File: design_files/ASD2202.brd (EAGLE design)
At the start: 22.5 x 21.3 mm, 21 parts, among them J1 DF12-32-DP, J2 DF12-32-DS, U1 XC6217A332MR-G, U2 24FC1025T-I/SN, U4 TXB0104, U5 W25Q80DVSNIG, MB85RS1MTPNF, 2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

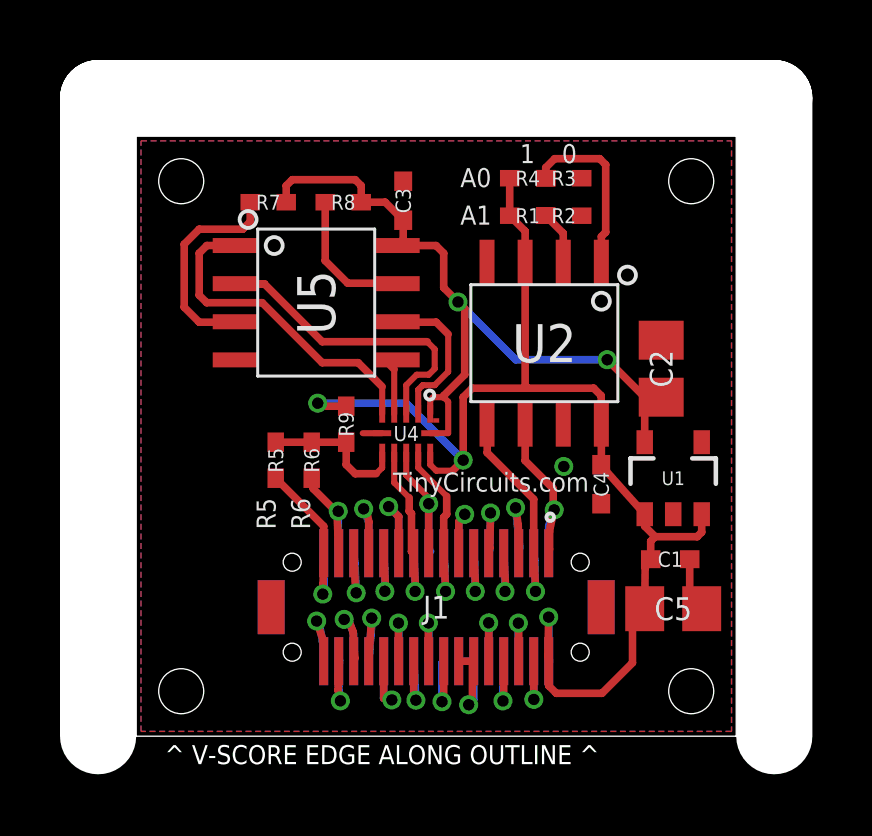
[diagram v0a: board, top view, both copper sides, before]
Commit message: update format
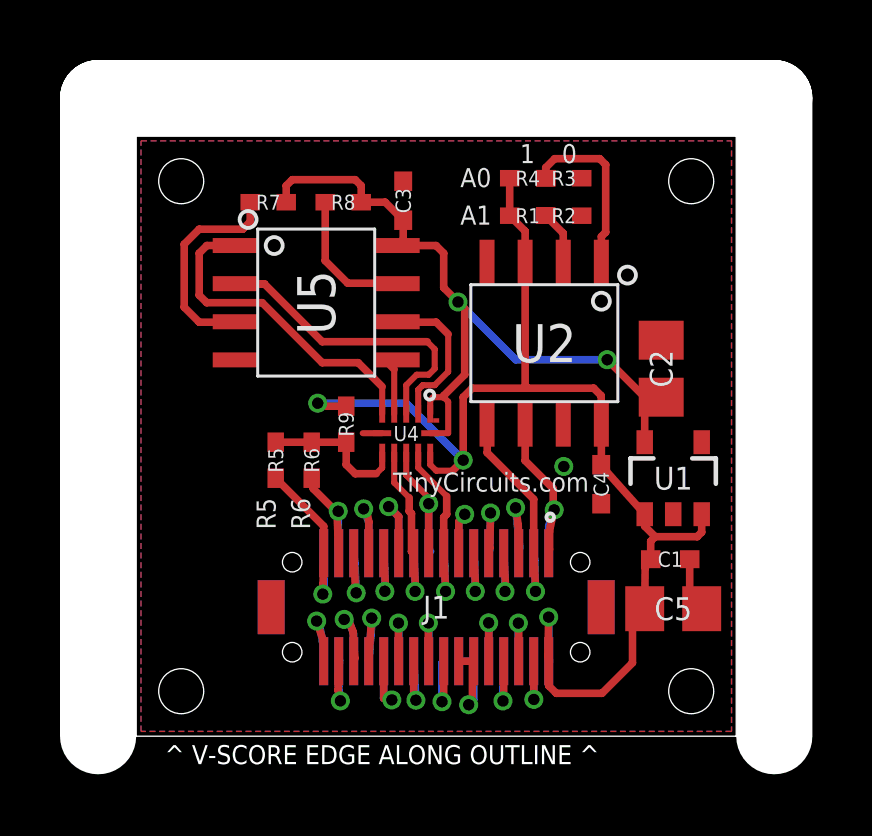
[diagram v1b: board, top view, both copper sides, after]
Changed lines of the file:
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@@
 <setting verticaltext="up"/>
 </settings>
-<grid distance="0.05" unitdist="mm" unit="mm" style="lines" multiple="1" display="yes" altdistance="0.025" altunitdist="inch" altunit="inch"/>
+<grid distance="0.1" unitdist="mm" unit="mm" style="lines" multiple="1" display="yes" altdistance="0.025" altunitdist="inch" altunit="inch"/>
 <layers>
 <layer number="1" name="Top" color="4" fill="1" visible="yes" active="yes"/>
@@
 <layer number="54" name="bGND_GNDA" color="7" fill="1" visible="yes" active="yes"/>
 <layer number="56" name="wert" color="7" fill="1" visible="yes" active="yes"/>
+<layer number="57" name="tCAD" color="7" fill="1" visible="no" active="no"/>
+<layer number="58" name="bCAD" color="7" fill="1" visible="no" active="no"/>
+<layer number="59" name="Invisible" color="7" fill="1" visible="no" active="no"/>
+<layer number="61" name="stand" color="7" fill="1" visible="no" active="no"/>
+<layer number="90" name="Modules" color="5" fill="1" visible="yes" active="yes"/>
 <layer number="91" name="Nets" color="2" fill="1" visible="no" active="no"/>
 <layer number="92" name="Busses" color="1" fill="1" visible="no" active="no"/>
@@
 <layer number="97" name="Info" color="7" fill="1" visible="no" active="no"/>
 <layer number="98" name="Guide" color="6" fill="1" visible="no" active="no"/>
+<layer number="99" name="SpiceOrder" color="5" fill="1" visible="no" active="no"/>
 <layer number="100" name="Muster" color="7" fill="1" visible="yes" active="yes"/>
 <layer number="101" name="Patch_Top" color="7" fill="1" visible="yes" active="yes"/>
@@
 <layer number="111" name="tGTest" color="4" fill="1" visible="no" active="no"/>
 <layer number="112" name="bGTest" color="1" fill="1" visible="no" active="no"/>
+<layer number="113" name="HENWAY_PKG" color="12" fill="1" visible="yes" active="yes"/>
+<layer number="114" name="50_Electronics_Plate" color="7" fill="1" visible="yes" active="yes"/>
+<layer number="115" name="henwayRES" color="5" fill="1" visible="yes" active="yes"/>
 <layer number="116" name="Patch_BOT" color="7" fill="1" visible="yes" active="yes"/>
 <layer number="117" name="mPads" color="7" fill="1" visible="no" active="no"/>
@@
 <layer number="151" name="HeatSink" color="7" fill="1" visible="yes" active="yes"/>
 <layer number="152" name="mbDocu" color="7" fill="1" visible="no" active="no"/>
+<layer number="153" name="FabDoc1" color="6" fill="1" visible="no" active="no"/>
+<layer number="154" name="FabDoc2" color="2" fill="1" visible="no" active="no"/>
+<layer number="155" name="FabDoc3" color="7" fill="15" visible="no" active="no"/>
+<layer number="156" name="bCapacitor" color="7" fill="1" visible="no" active="yes"/>
+<layer number="157" name="tResistor" color="7" fill="1" visible="no" active="yes"/>
+<layer number="158" name="bResistor" color="7" fill="1" visible="no" active="yes"/>
+<layer number="159" name="henwayCAP" color="13" fill="1" visible="yes" active="yes"/>
 <layer number="191" name="mNets" color="7" fill="1" visible="no" active="no"/>
 <layer number="192" name="mBusses" color="7" fill="1" visible="no" active="no"/>
@@
 <layer number="223" name="223bmp" color="7" fill="1" visible="yes" active="yes"/>
 <layer number="224" name="224bmp" color="7" fill="1" visible="yes" active="yes"/>
+<layer number="231" name="Eagle3D_PG1" color="7" fill="1" visible="yes" active="yes"/>
+<layer number="232" name="Eagle3D_PG2" color="7" fill="1" visible="yes" active="yes"/>
+<layer number="233" name="Eagle3D_PG3" color="7" fill="1" visible="yes" active="yes"/>
 <layer number="248" name="Housing" color="7" fill="1" visible="yes" active="yes"/>
 <layer number="249" name="Edge" color="7" fill="1" visible="yes" active="yes"/>
@@
 <attribute name="PARTNO" value="AS-ITM-00249" x="27.9" y="18.6" size="1.778" layer="27" display="off"/>
 <attribute name="VALUE" value="XC6217A33" x="27.9" y="18.6" size="1.778" layer="27" display="off"/>
+<attribute name="PNPROTATION" value="270" x="27.9" y="18.6" size="1.778" layer="27" display="off"/>
 </element>
 <element name="U4" library="tinycircuits" package="UQFN-12" value="TXB0104" x="19" y="20.1" rot="R180">
 <attribute name="PARTNO" value="AS-ITM-00048" x="19" y="20.1" size="1.778" layer="27" rot="R180" display="off"/>
 <attribute name="VALUE" value="TXB0104" x="19" y="20.1" size="1.778" layer="27" rot="R180" display="off"/>
+<attribute name="PNPROTATION" value="0" x="19" y="20.1" size="1.778" layer="27" rot="R180" display="off"/>
 </element>
 <element name="R8" library="tinycircuits" package="0402" value="1.00K" x="16.9" y="27.8">
@@
 <attribute name="PARTNO" value="AS-ITM-00238" x="16" y="24.45" size="1.778" layer="27" rot="R270" display="off"/>
 <attribute name="VALUE" value="W25Q40BVSNIG" x="16" y="24.45" size="1.778" layer="27" rot="R270" display="off"/>
+<attribute name="PNPROTATION" value="90" x="16" y="24.45" size="1.778" layer="27" rot="R270" display="off"/>
 </element>
 </elements>
